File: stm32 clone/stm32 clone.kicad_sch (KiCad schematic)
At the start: 18 parts, among them J1 DEBUG, J2 USB_C_Receptacle_USB2.0_16P, SW1 RST, U1 STM32G030C6T6, Y1 8 MHz, Y2 32.768 KHz

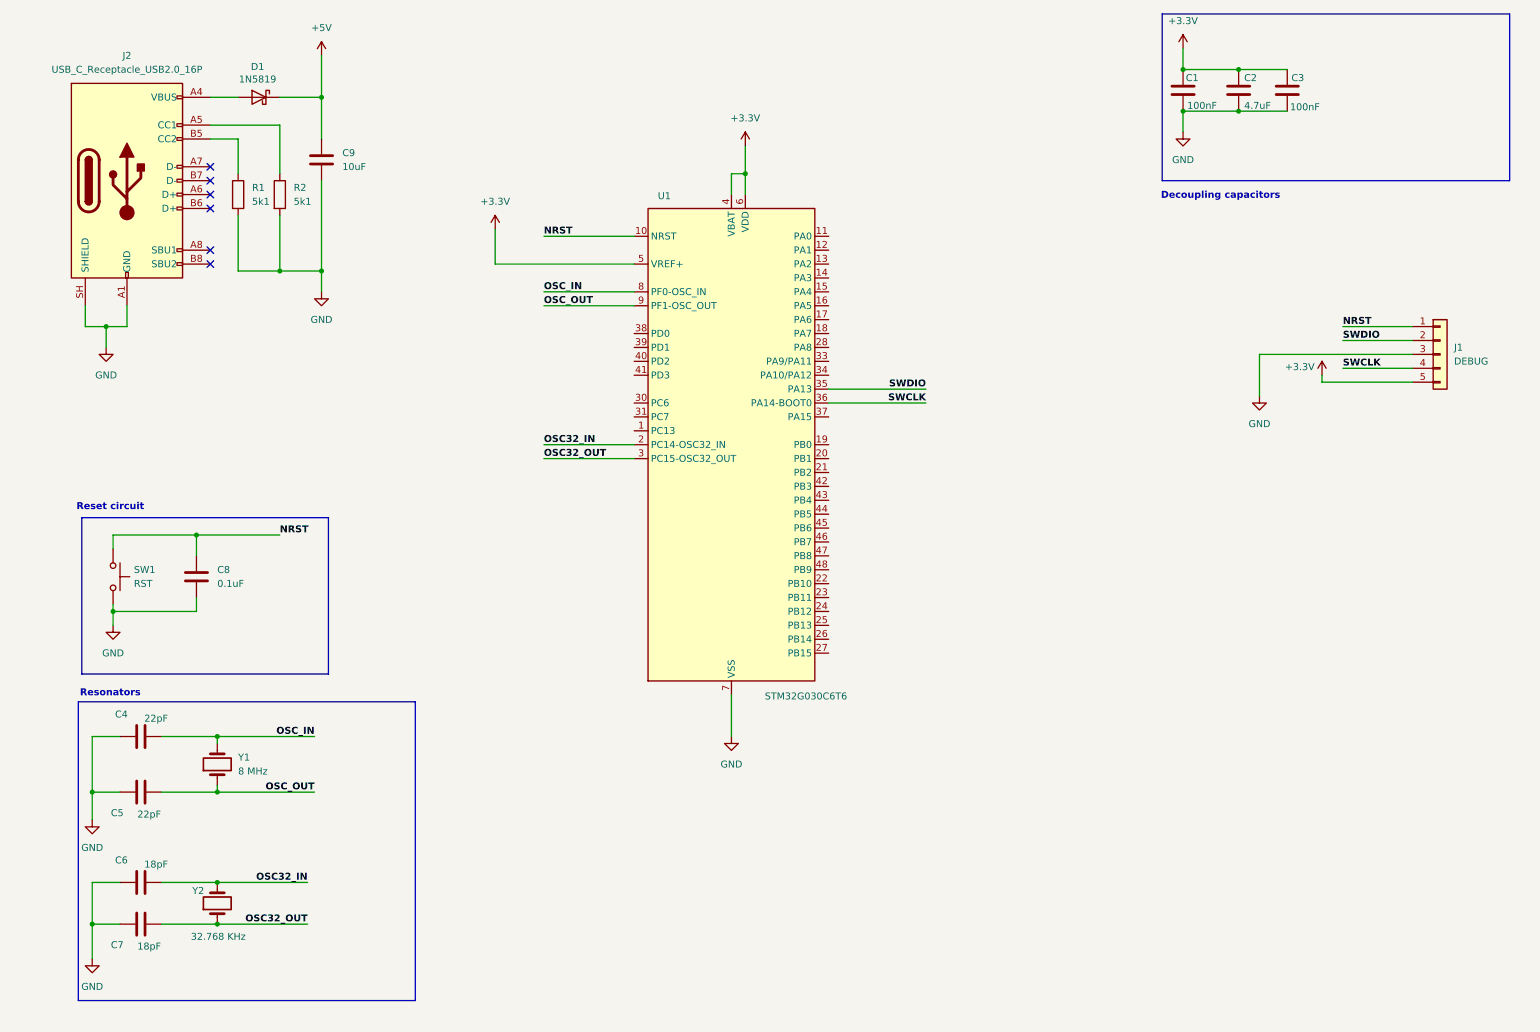
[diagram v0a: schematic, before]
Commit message: usb finished
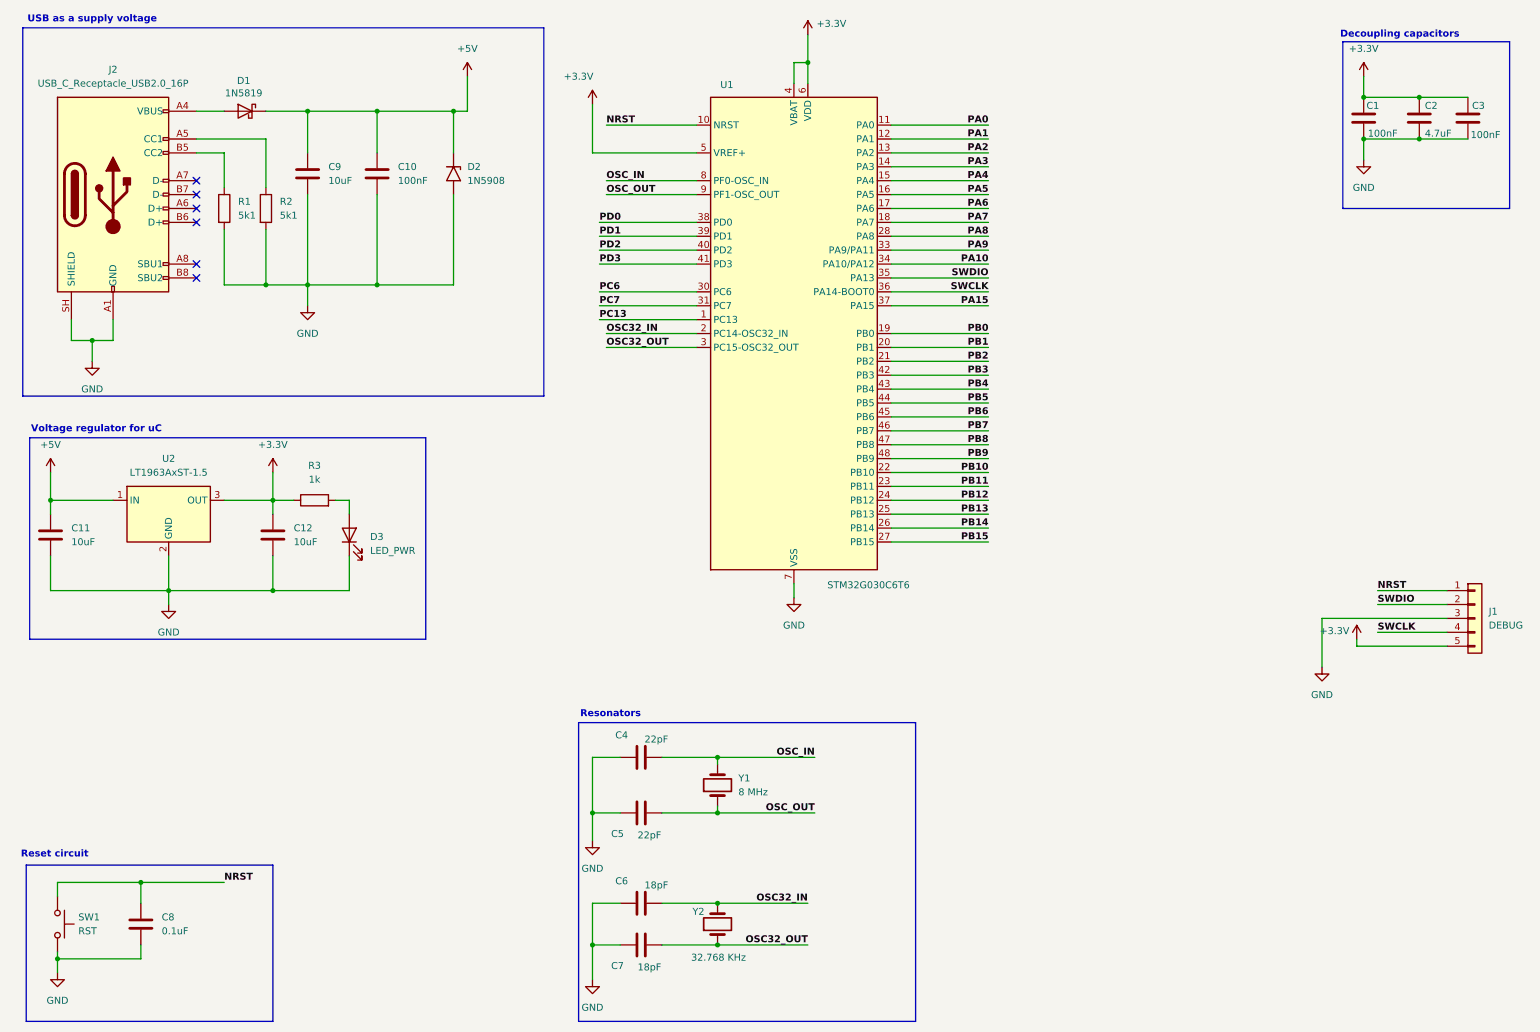
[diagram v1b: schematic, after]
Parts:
- added C10: 100nF, Capacitor_SMD:C_0805_2012Metric_Pad1.18x1.45mm_HandSolder, symbol Device:C
- added C11, C12: 10uF, Capacitor_SMD:C_0805_2012Metric_Pad1.18x1.45mm_HandSolder, symbol Device:C
- added D2: 1N5908, Diode_THT:D_DO-201AE_P15.24mm_Horizontal, symbol Diode:1N62xxA
- added D3: LED_PWR, LED_THT:LED_D5.0mm, symbol Device:LED
- added R3: 1k, symbol Device:R
- added U2: LT1963AxST-1.5, Package_TO_SOT_SMD:SOT-223-3_TabPin2, symbol Regulator_Linear:LT1963AxST-1.5
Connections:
- net +3.3V: now also C12.1, R3.1, U2.3 (OUT)
- net +5V: now also C10.1, C11.1, D2.1 (A1), U2.1 (IN)
- net GND: now also C10.2, C11.2, C12.2, D2.2 (A2), D3.1 (K), U2.2 (GND)
- net PC13: now reaches U1.1 (PC13)
- net PA0: now reaches U1.11 (PA0)
- net PA1: now reaches U1.12 (PA1)
- net PA2: now reaches U1.13 (PA2)
- net PA3: now reaches U1.14 (PA3)
- net PA4: now reaches U1.15 (PA4)
- net PA5: now reaches U1.16 (PA5)
- net PA6: now reaches U1.17 (PA6)
- net PA7: now reaches U1.18 (PA7)
- net PB0: now reaches U1.19 (PB0)
- net PB1: now reaches U1.20 (PB1)
- net PB2: now reaches U1.21 (PB2)
- net PB10: now reaches U1.22 (PB10)
- net PB11: now reaches U1.23 (PB11)
- net PB12: now reaches U1.24 (PB12)
- net PB13: now reaches U1.25 (PB13)
- net PB14: now reaches U1.26 (PB14)
- net PB15: now reaches U1.27 (PB15)
- net PA8: now reaches U1.28 (PA8)
- net PC6: now reaches U1.30 (PC6)
- net PC7: now reaches U1.31 (PC7)
- net PA9: now reaches U1.33 (PA9/PA11)
- net PA10: now reaches U1.34 (PA10/PA12)
- net PA15: now reaches U1.37 (PA15)
- net PD0: now reaches U1.38 (PD0)
- net PD1: now reaches U1.39 (PD1)
- net PD2: now reaches U1.40 (PD2)
- net PD3: now reaches U1.41 (PD3)
- net PB3: now reaches U1.42 (PB3)
- net PB4: now reaches U1.43 (PB4)
- net PB5: now reaches U1.44 (PB5)
- net PB6: now reaches U1.45 (PB6)
- net PB7: now reaches U1.46 (PB7)
- net PB8: now reaches U1.47 (PB8)
- net PB9: now reaches U1.48 (PB9)
- new net: D3.2 (A), R3.2
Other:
- note added: "USB as a supply voltage"
- note added: "Voltage regulator for uC"
- moved on the sheet: C1, C2, C3, C4, C5, C6, C7, C8, C9, D1, J1, J2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
